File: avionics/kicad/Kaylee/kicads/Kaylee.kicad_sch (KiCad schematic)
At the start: 142 parts

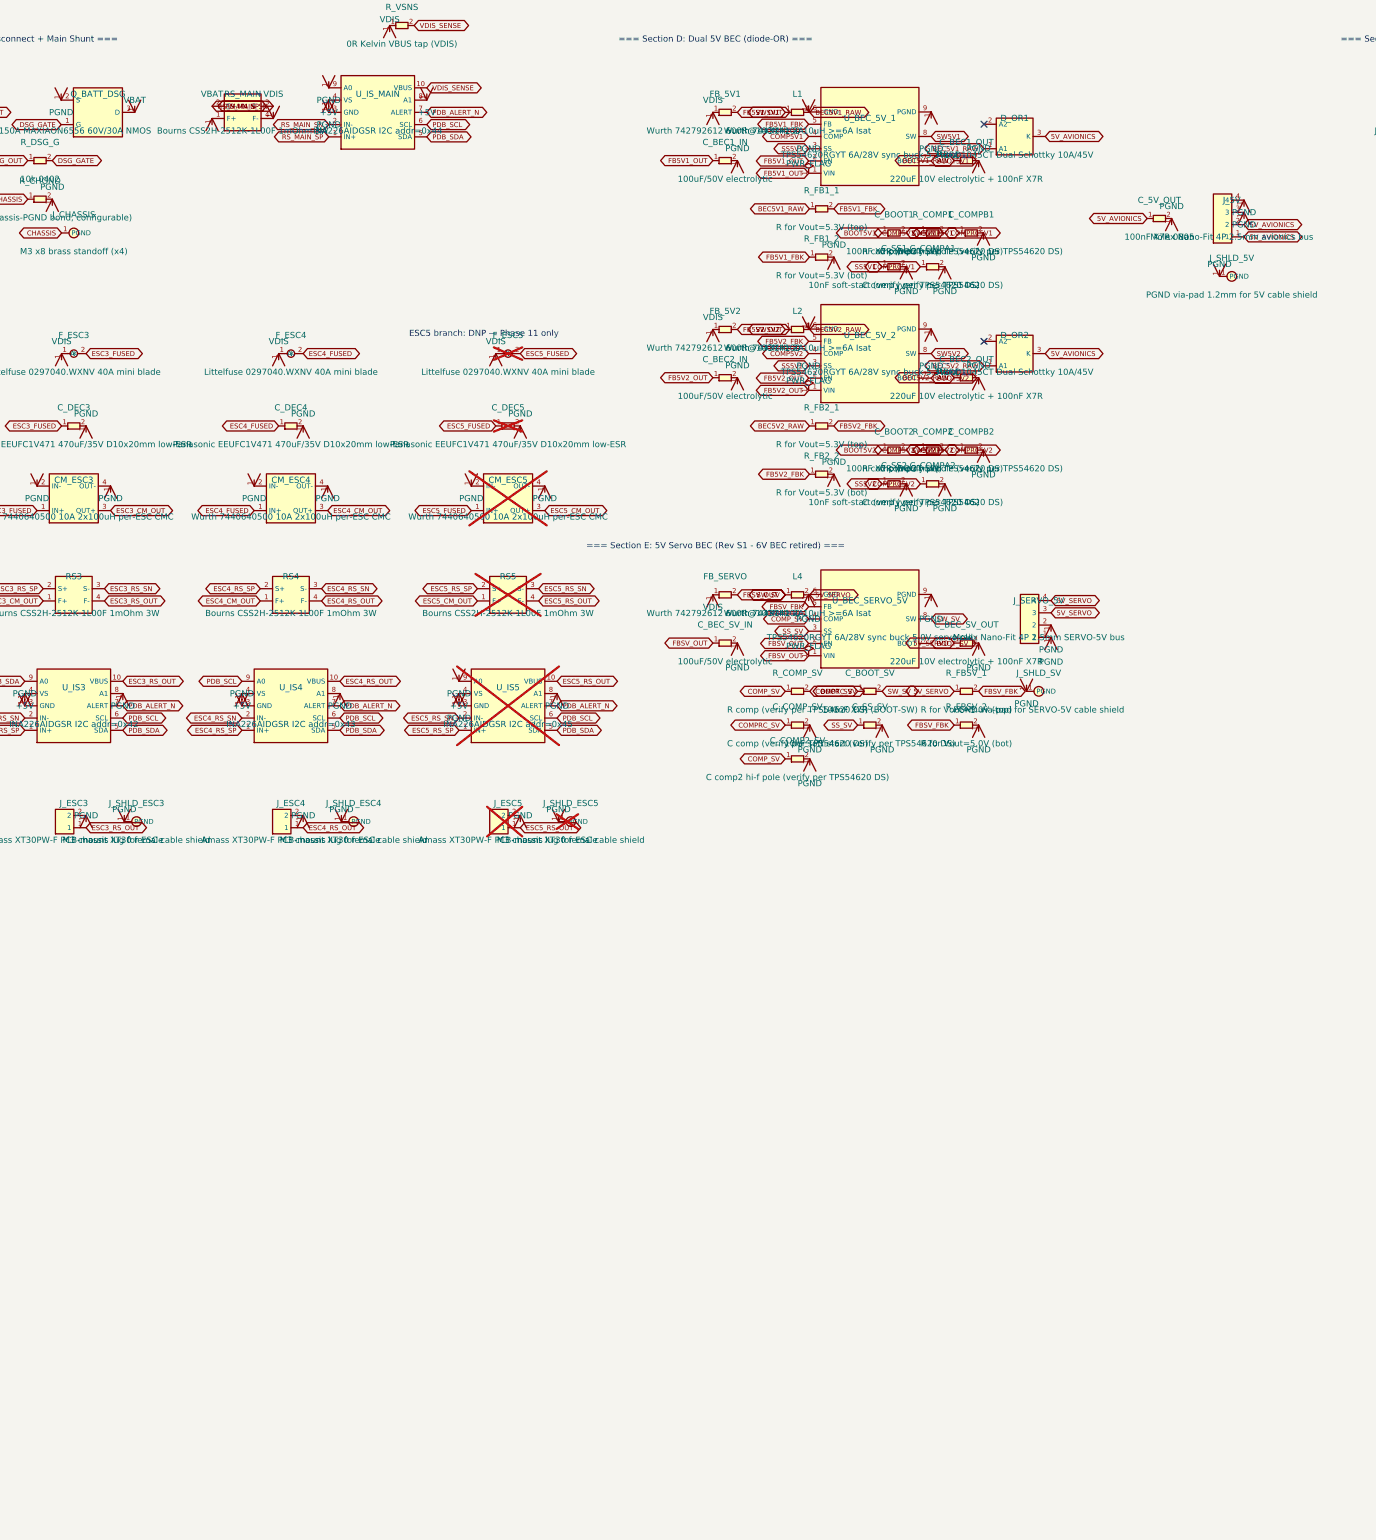
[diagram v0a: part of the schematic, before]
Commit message: wash kaylee and firmware
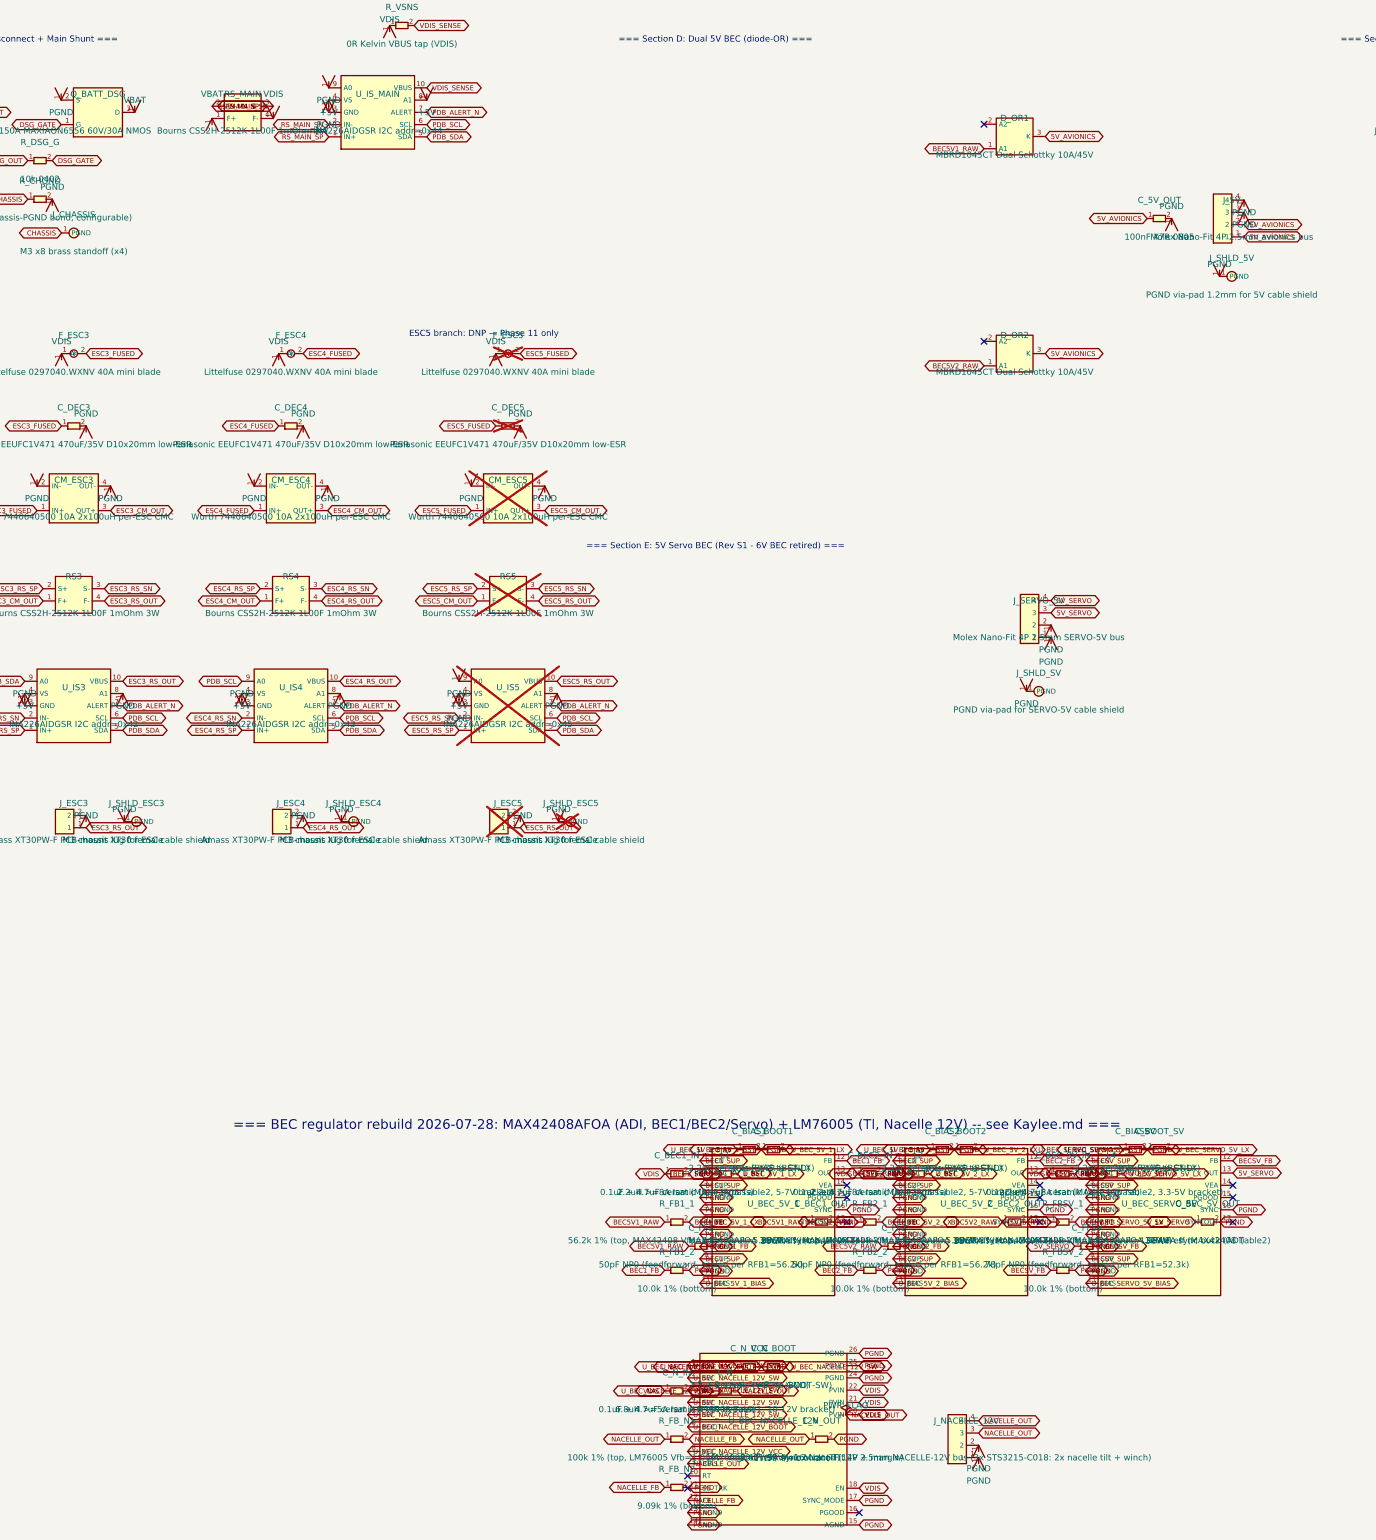
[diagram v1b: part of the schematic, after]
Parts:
- removed C_COMP2_SV, C_COMPB1, C_COMPB2: C comp2 hi-f pole (verify per TPS54620 DS), symbol C_Generic
- removed C_COMPA1, C_COMPA2, C_COMP_SV: C comp (verify per TPS54620 DS), symbol C_Generic
- removed C_SS1, C_SS2, C_SS_SV: 10nF soft-start (verify per TPS54620 DS), symbol C_Generic
- removed FB_5V1, FB_5V2, FB_SERVO: Wurth 742792612 600R@100MHz 2A, symbol FB_Generic
- removed R_COMP1, R_COMP2, R_COMP_SV: R comp (verify per TPS54620 DS), symbol R_Generic
- removed U_BEC_5V_1, U_BEC_5V_2: TPS54620RGYT 6A/28V sync buck 5.3Vout, symbol TPS54620RGYT
- removed U_BEC_SERVO_5V: TPS54620RGYT 6A/28V sync buck 5.0V servo rail, symbol TPS54620RGYT
- added C_BIAS1, C_BIAS2, C_BIASSV: 2.2uF ceramic (BIAS to GND), symbol C_Generic
- added C_FF1, C_FF2: 50pF NP0 (feedforward, scaled per RFB1=56.2k), symbol C_Generic
- added C_FFSV: 78pF NP0 (feedforward, scaled per RFB1=52.3k), symbol C_Generic
- added C_N_BOOT: 0.47uF, >=6.3V (BOOT-SW), symbol C_Generic
- added C_N_IN: 0.1uF + 4.7uF ceramic (PVIN bypass), symbol C_Generic
- added C_N_OUT: 90uF eff, >=16V rated (12V + margin), symbol C_Generic
- added C_N_VCC: 2.2uF ceramic (VCC to GND), symbol C_Generic
- added J_NACELLE_12V: Molex Nano-Fit 4P 2.5mm NACELLE-12V bus (3x STS32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, symbol Nano_Fit_4P
- added L_N: 6.8uH >=5A Isat (LM76005 Table1, 10-12V bracket), symbol L_Generic
- added R_FB_N1: 100k 1% (top, LM76005 Vfb=1.006V, Vout=11.99V), symbol R_Generic
- added R_FB_N2: 9.09k 1% (bottom), symbol R_Generic
- added U_BEC_5V_1, U_BEC_5V_2, U_BEC_SERVO_5V: MAX42408AFOA 36V/8A sync buck (ADI), Kaylee:MAX42408AFOA_FC2QFN17_3.5x3.75mm, symbol MAX42408AFOA
- added U_BEC_NACELLE_12V: LM76005 60V/5A sync buck (TI), Package_DFN_QFN:Texas_RNP0030B_WQFN-30-1EP_4x6mm_P0.5mm_EP1.8x4.5mm, symbol LM76005
- C_BEC1_IN, C_BEC2_IN, C_BEC_SV_IN: value 100uF/50V electrolytic -> 0.1uF + 4.7uF ceramic (SUP bypass)
- C_BEC1_OUT, C_BEC2_OUT: value 220uF 10V electrolytic + 100nF X7R -> 88uF eff (MAX42408 Table2)
- C_BEC_SV_OUT: value 220uF 10V electrolytic + 100nF X7R -> 120uF eff (MAX42408 Table2)
- C_BOOT1, C_BOOT2, C_BOOT_SV: value 100nF X7R (BOOT-SW) -> 0.1uF X7R (BST-LX)
- L1, L2: value Wurth 744314100 10uH >=6A Isat -> 2.2uH >=8A Isat (MAX42408 Table2, 5-7V bracket)
- L4: value Wurth 744314100 10uH >=6A Isat -> 2.2uH >=8A Isat (MAX42408 Table2, 3.3-5V bracket)
- R_FB1_1, R_FB2_1: value R for Vout=5.3V (top) -> 56.2k 1% (top, MAX42408 Vfb=0.8V, Vout=5.296V)
- R_FB1_2, R_FB2_2: value R for Vout=5.3V (bot) -> 10.0k 1% (bottom)
- R_FBSV_1: value R for Vout=5.0V (top) -> 52.3k 1% (top, MAX42408 Vfb=0.8V, Vout=4.984V)
- R_FBSV_2: value R for Vout=5.0V (bot) -> 10.0k 1% (bottom)
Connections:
- net FB5V1_OUT is gone; now on net VDIS: C_BEC1_IN.1
- net FB5V2_OUT is gone; now on net VDIS: C_BEC2_IN.1
- net FBSV_OUT is gone; now on net VDIS: C_BEC_SV_IN.1
- net 5V_SERVO: now also C_FFSV.1, U_BEC_SERVO_5V.13 (OUT); no longer L4.2
- net BEC5V1_RAW: now also C_FF1.1, U_BEC_5V_1.13 (OUT); no longer L1.2
- net BEC5V2_RAW: now also C_FF2.1, U_BEC_5V_2.13 (OUT); no longer L2.2
- net PGND: now also C_BIAS1.2, C_BIAS2.2, C_BIASSV.2, C_N_IN.2, C_N_OUT.2, C_N_VCC.2, J_NACELLE_12V.1, J_NACELLE_12V.2, R_FB_N2.2, U_BEC_5V_1.10 (GND), U_BEC_5V_1.16 (SYNC), U_BEC_5V_1.4 (PGND), U_BEC_5V_1.5 (PGND), U_BEC_5V_1.7 (PGND), U_BEC_5V_1.8 (PGND), U_BEC_5V_2.10 (GND), U_BEC_5V_2.16 (SYNC), U_BEC_5V_2.4 (PGND), U_BEC_5V_2.5 (PGND), U_BEC_5V_2.7 (PGND), U_BEC_5V_2.8 (PGND), U_BEC_NACELLE_12V.13 (AGND), U_BEC_NACELLE_12V.14 (AGND), U_BEC_NACELLE_12V.15 (AGND), U_BEC_NACELLE_12V.17 (SYNC_MODE), U_BEC_NACELLE_12V.24 (PGND), U_BEC_NACELLE_12V.25 (PGND), U_BEC_NACELLE_12V.26 (PGND), U_BEC_SERVO_5V.10 (GND), U_BEC_SERVO_5V.16 (SYNC), U_BEC_SERVO_5V.4 (PGND), U_BEC_SERVO_5V.5 (PGND), U_BEC_SERVO_5V.7 (PGND), U_BEC_SERVO_5V.8 (PGND)
- net VDIS: now also C_N_IN.1, U_BEC_NACELLE_12V.18 (EN), U_BEC_NACELLE_12V.20 (PVIN), U_BEC_NACELLE_12V.21 (PVIN), U_BEC_NACELLE_12V.22 (PVIN)
- net BOOT5V1 renamed U_BEC_5V_1_BST
- net U_BEC_5V_1_BST: now also U_BEC_5V_1.2 (BST)
- net BOOT5V2 renamed U_BEC_5V_2_BST
- net U_BEC_5V_2_BST: now also U_BEC_5V_2.2 (BST)
- net BOOT_SV renamed U_BEC_SERVO_5V_BST
- net U_BEC_SERVO_5V_BST: now also U_BEC_SERVO_5V.2 (BST)
- net FB5V1_FBK renamed BEC1_FB
- net BEC1_FB: now also C_FF1.2, U_BEC_5V_1.12 (FB)
- net FB5V2_FBK renamed BEC2_FB
- net BEC2_FB: now also C_FF2.2, U_BEC_5V_2.12 (FB)
- net FBSV_FBK renamed BECSV_FB
- net BECSV_FB: now also C_FFSV.2, U_BEC_SERVO_5V.12 (FB)
- net SW5V1 renamed BEC1_SUP
- net BEC1_SUP: now also U_BEC_5V_1.1 (EN), U_BEC_5V_1.3 (SUP), U_BEC_5V_1.9 (SUP); no longer C_BOOT1.2
- net SW5V2 renamed BEC2_SUP
- net BEC2_SUP: now also U_BEC_5V_2.1 (EN), U_BEC_5V_2.3 (SUP), U_BEC_5V_2.9 (SUP); no longer C_BOOT2.2
- net SW_SV renamed BECSV_SUP
- net BECSV_SUP: now also U_BEC_SERVO_5V.1 (EN), U_BEC_SERVO_5V.3 (SUP), U_BEC_SERVO_5V.9 (SUP); no longer C_BOOT_SV.2
- new net NACELLE_FB: R_FB_N1.2, R_FB_N2.1, U_BEC_NACELLE_12V.12 (FB)
- new net NACELLE_OUT: C_N_OUT.1, J_NACELLE_12V.3, J_NACELLE_12V.4, L_N.2, R_FB_N1.1, U_BEC_NACELLE_12V.9 (BIAS)
- new net U_BEC_5V_1_BIAS: C_BIAS1.1, U_BEC_5V_1.11 (BIAS)
- new net U_BEC_5V_1_LX: C_BOOT1.2, L1.2, U_BEC_5V_1.6 (LX)
- new net U_BEC_5V_2_BIAS: C_BIAS2.1, U_BEC_5V_2.11 (BIAS)
- new net U_BEC_5V_2_LX: C_BOOT2.2, L2.2, U_BEC_5V_2.6 (LX)
- new net U_BEC_NACELLE_12V_BOOT: C_N_BOOT.1, U_BEC_NACELLE_12V.6 (BOOT)
- new net U_BEC_NACELLE_12V_SW: C_N_BOOT.2, L_N.1, U_BEC_NACELLE_12V.1 (SW), U_BEC_NACELLE_12V.2 (SW), U_BEC_NACELLE_12V.3 (SW), U_BEC_NACELLE_12V.4 (SW), U_BEC_NACELLE_12V.5 (SW)
- new net U_BEC_NACELLE_12V_VCC: C_N_VCC.1, U_BEC_NACELLE_12V.8 (VCC)
- new net U_BEC_SERVO_5V_BIAS: C_BIASSV.1, U_BEC_SERVO_5V.11 (BIAS)
- new net U_BEC_SERVO_5V_LX: C_BOOT_SV.2, L4.2, U_BEC_SERVO_5V.6 (LX)
- no-connect marks 55 -> 67
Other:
- note added: "=== BEC regulator rebuild 2026-07-28: MAX42408AFOA (ADI, BEC1/BEC2/Servo) + LM76005 (TI, Nacelle 12V) -- see Kaylee.md ==="
